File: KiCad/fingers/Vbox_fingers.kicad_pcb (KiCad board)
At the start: 2 copper layers, 33.1 x 114.3 mm, 4 parts, among them J4 Conn_01x06, J5 Conn_01x06, J6 Conn_01x10, J7 Conn_01x10

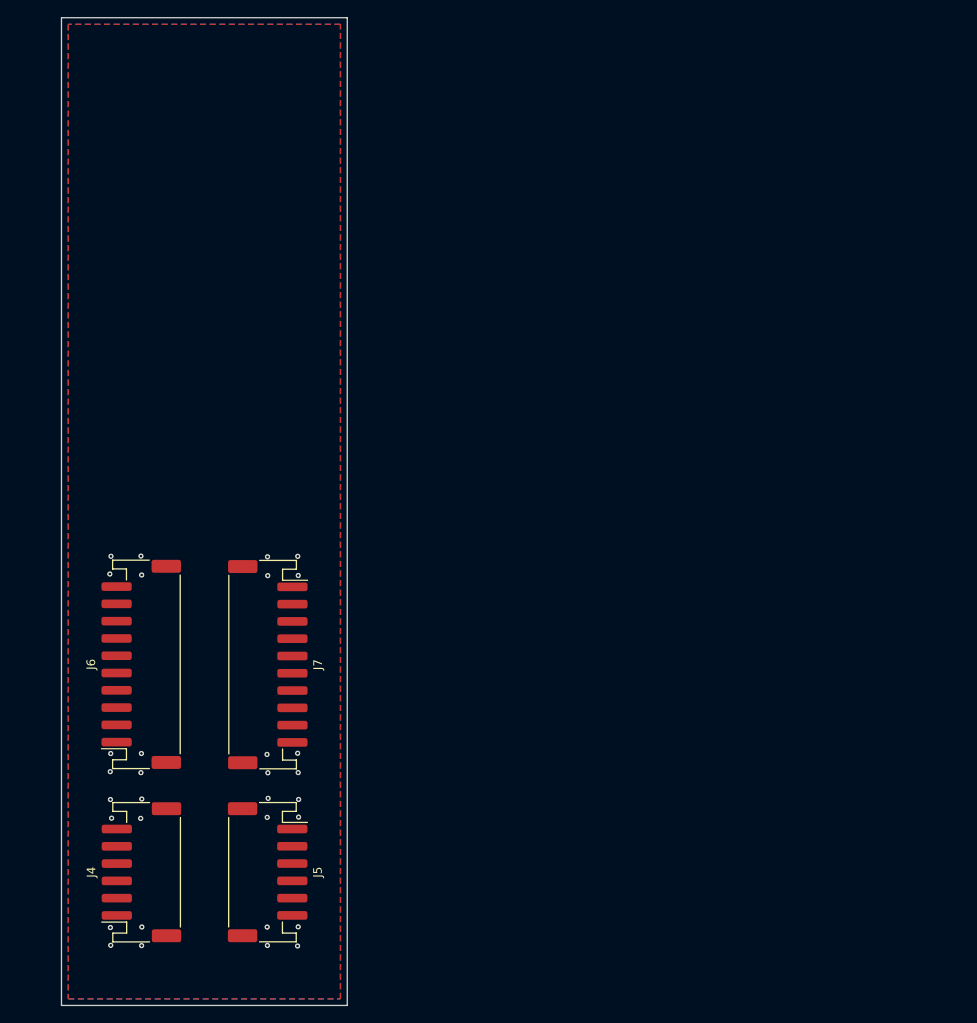
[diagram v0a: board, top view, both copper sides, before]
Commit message: thumbs and fingers
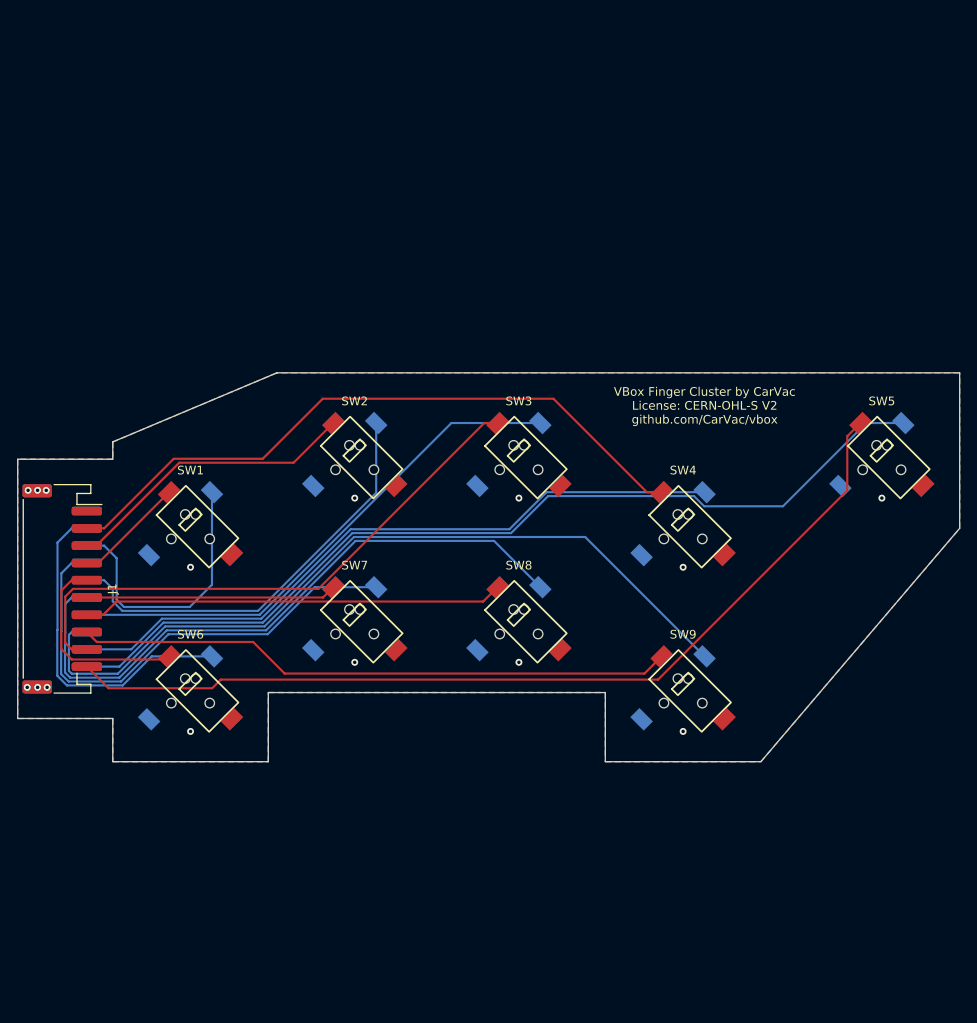
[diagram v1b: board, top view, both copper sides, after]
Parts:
- removed J4, J5: Conn_01x06, Connector_JST:JST_PH_S6B-PH-SM4-TB_1x06-1MP_P2.00mm_Horizontal
- removed J6, J7: Conn_01x10, Connector_JST:JST_PH_S10B-PH-SM4-TB_1x10-1MP_P2.00mm_Horizontal
- added J1: Conn_01x10, Connector_JST:JST_PH_S10B-PH-SM4-TB_1x10-1MP_P2.00mm_Horizontal, F.Cu at (85.2, 108.0)
- added J2: Conn_01x10, Connector_JST:JST_PH_S10B-PH-SM4-TB_1x10-1MP_P2.00mm_Horizontal, B.Cu at (85.2, 108.0)
- added SW1: SW_Push_45deg, Buttons:Vbox, F.Cu at (100.0, 100.0)
- added SW10: SW_Push_45deg, Buttons:Vbox, B.Cu at (100.0, 100.0)
- added SW11: SW_Push_45deg, Buttons:Vbox, B.Cu at (119.0, 92.0)
- added SW12: SW_Push_45deg, Buttons:Vbox, B.Cu at (138.0, 92.0)
- added SW13: SW_Push_45deg, Buttons:Vbox, B.Cu at (157.0, 100.0)
- added SW14: SW_Push_45deg, Buttons:Vbox, B.Cu at (180.0, 92.0)
- added SW15: SW_Push_45deg, Buttons:Vbox, B.Cu at (100.0, 119.0)
- added SW16: SW_Push_45deg, Buttons:Vbox, B.Cu at (119.0, 111.0)
- added SW17: SW_Push_45deg, Buttons:Vbox, B.Cu at (138.0, 111.0)
- added SW18: SW_Push_45deg, Buttons:Vbox, B.Cu at (157.0, 119.0)
- added SW2: SW_Push_45deg, Buttons:Vbox, F.Cu at (119.0, 92.0)
- added SW3: SW_Push_45deg, Buttons:Vbox, F.Cu at (138.0, 92.0)
- added SW4: SW_Push_45deg, Buttons:Vbox, F.Cu at (157.0, 100.0)
- added SW5: SW_Push_45deg, Buttons:Vbox, F.Cu at (180.0, 92.0)
- added SW6: SW_Push_45deg, Buttons:Vbox, F.Cu at (100.0, 119.0)
- added SW7: SW_Push_45deg, Buttons:Vbox, F.Cu at (119.0, 111.0)
- added SW8: SW_Push_45deg, Buttons:Vbox, F.Cu at (138.0, 111.0)
- added SW9: SW_Push_45deg, Buttons:Vbox, F.Cu at (157.0, 119.0)
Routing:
- net RIGHTSTART: track 0.00 -> 107.1 mm
- net START: track 0.00 -> 106.9 mm
- net B: track 0.00 -> 92.3 mm
- net R: track 0.00 -> 79.0 mm
- net INDEX2: track 0.00 -> 77.2 mm
- net X: track 0.00 -> 74.8 mm
- net RIGHT: track 0.00 -> 69.3 mm
- net UP2: track 0.00 -> 66.5 mm
- net Y: track 0.00 -> 61.7 mm
- net Z: track 0.00 -> 56.5 mm
- net LS: track 0.00 -> 49.5 mm
- net DOWN: track 0.00 -> 48.8 mm
- net UP: track 0.00 -> 39.3 mm
- net RING2: track 0.00 -> 34.4 mm
- net MS: track 0.00 -> 32.0 mm
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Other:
- board size 33.1 x 114.3 mm -> 109 x 45 mm
- board text added: "VBox Finger Cluster by CarVac License: CERN-OHL-S V2 github.com/CarVac/vbox"
